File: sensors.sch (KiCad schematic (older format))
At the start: 77 parts, among them SW1 MicroSwitch, SW10 MicroSwitch, SW11 MicroSwitch, SW12 MicroSwitch, SW13 MicroSwitch, SW14 MicroSwitch, SW15 MicroSwitch, SW16 MicroSwitch, SW2 MicroSwitch, SW3 MicroSwitch, SW4 MicroSwitch, SW5 MicroSwitch, SW6 MicroSwitch, SW7 MicroSwitch, SW8 MicroSwitch, SW9 MicroSwitch, U5 BQ32000, X2 32768Hz

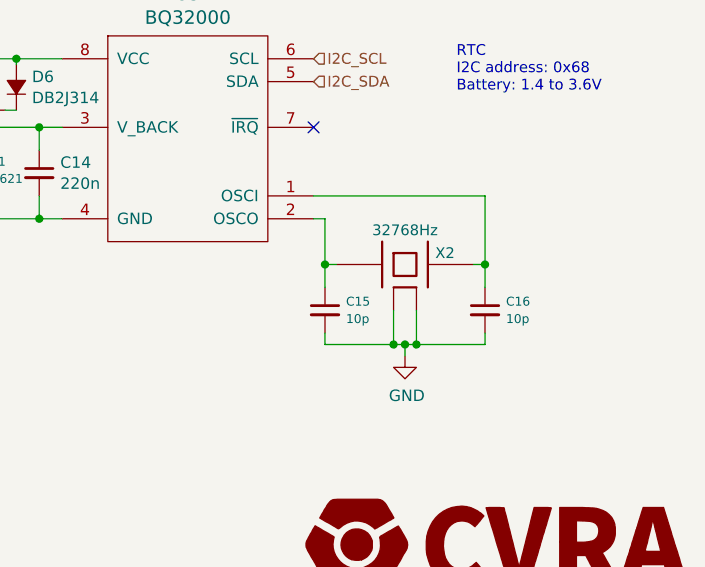
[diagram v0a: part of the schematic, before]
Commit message: Place components on PCB
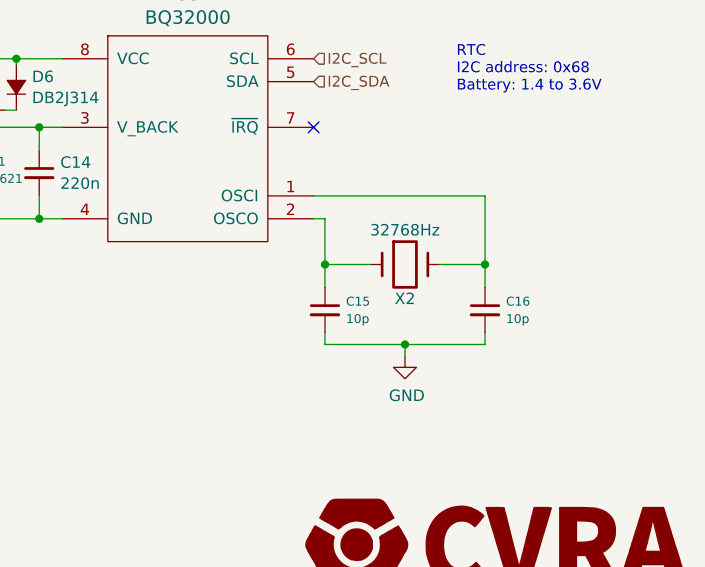
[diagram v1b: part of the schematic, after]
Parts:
- removed X2: 32768Hz, _div:XTAL_ABS07, symbol XTAL-SMD-4-PADS
- added X2: 32768Hz, _div:XTAL_ABS07, symbol Crystal
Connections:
- net at C16.1, U5.1 (OSCI): now also X2.2
- net at C15.1, U5.2 (OSCO): now also X2.1
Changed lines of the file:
@@
 	9425 5300 10175 5300
 Wire Wire Line
-	9525 5600 9475 5600
+	9675 5600 9475 5600
 Wire Wire Line
 	9475 5400 9475 5700
@@
 	1    0    0    -1
 $EndComp
-$Comp
-L XTAL-SMD-4-PADS X2
-U 1 1 56B4F654
-P 9825 5600
-F 0 "X2" H 10000 5650 47  0000 C CNN
-F 1 "32768Hz" H 9825 5750 47  0000 C CNN
-F 2 "_div:XTAL_ABS07" H 9825 5600 60  0001 C CNN
-F 3 "" H 9825 5600 60  0000 C CNN
-	1    9825 5600
-	1    0    0    -1
-$EndComp
 Wire Wire Line
 	10175 5300 10175 5700
 Wire Wire Line
-	10175 5600 10125 5600
+	10175 5600 9975 5600
 Connection ~ 10175 5600
 Wire Wire Line
@@
 	10175 5950 10175 5900
 Connection ~ 9825 5950
-Wire Wire Line
-	9875 5950 9875 5800
-Connection ~ 9875 5950
-Wire Wire Line
-	9775 5800 9775 5950
-Connection ~ 9775 5950
 $Comp
 L C_Small C14
@@
 Connection ~ 7550 4700
 Connection ~ 8125 4700
+$Comp
+L Crystal X2
+U 1 1 56D345FF
+P 9825 5600
+F 0 "X2" H 9825 5450 50  0000 C CNN
+F 1 "32768Hz" H 9825 5750 50  0000 C CNN
+F 2 "_div:XTAL_ABS07" H 9825 5600 50  0001 C CNN
+F 3 "" H 9825 5600 50  0000 C CNN
+	1    9825 5600
+	1    0    0    -1
+$EndComp
 $EndSCHEMATC
